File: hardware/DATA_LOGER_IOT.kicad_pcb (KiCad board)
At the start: 2 copper layers, 50 x 50 mm, 9 parts

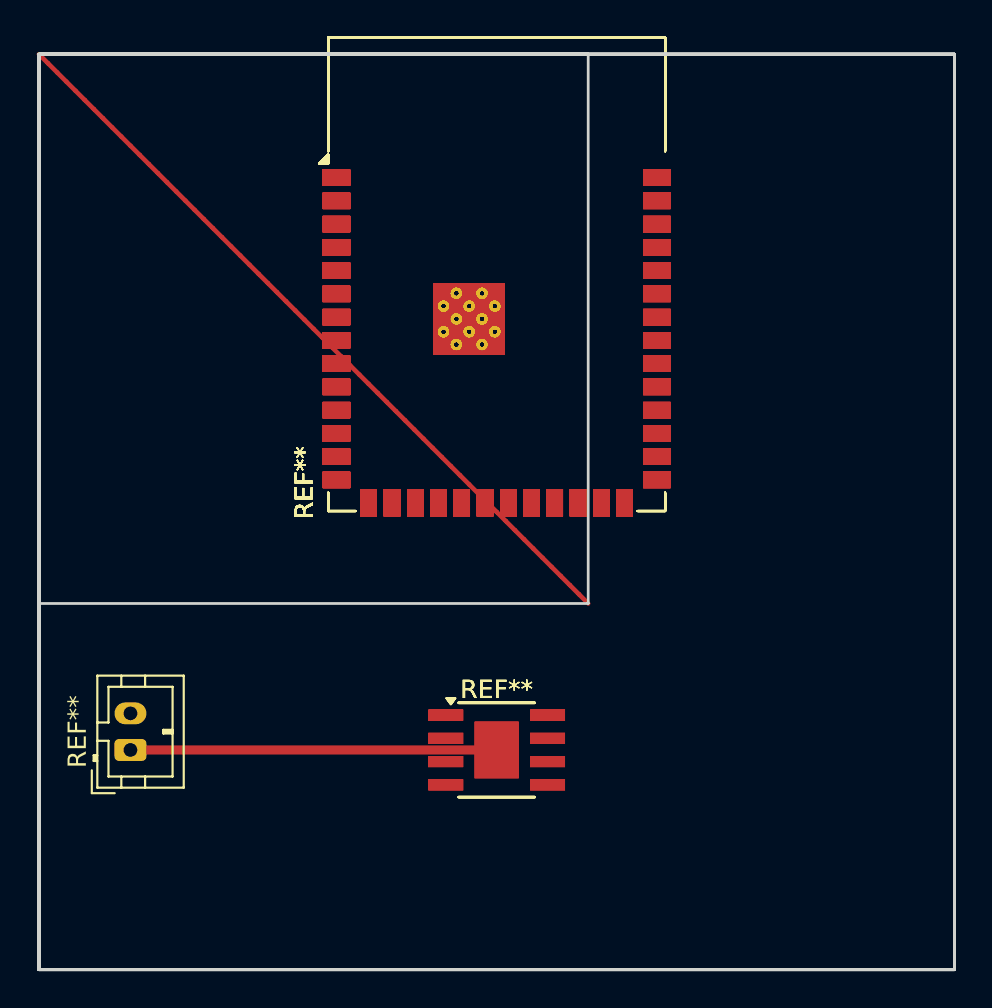
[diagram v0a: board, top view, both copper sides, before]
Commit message: WIP: guardar cambios antes de pull
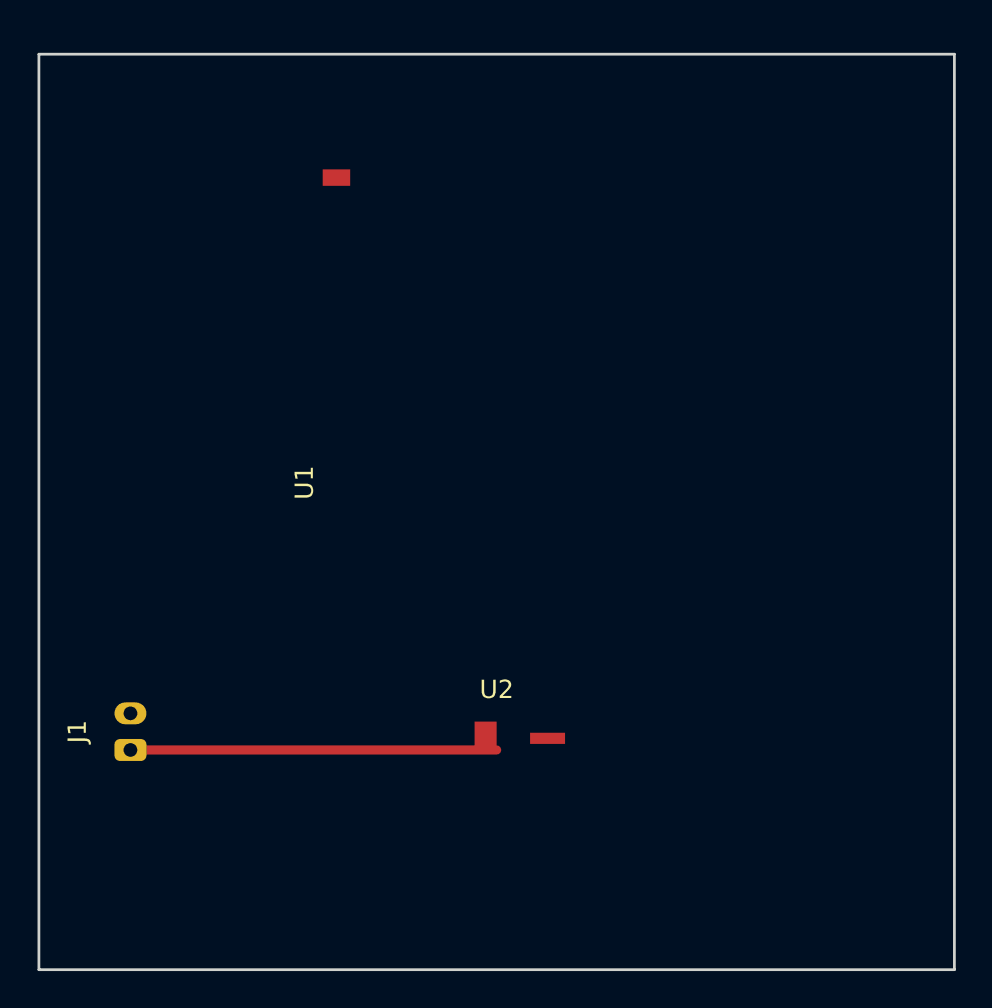
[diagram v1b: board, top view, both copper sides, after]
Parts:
- removed REF** (x5): ESP32-S3-WROOM-1, ESP32-S3-WROOM-1
- removed REF**: TI_SO-PowerPAD-8, TI_SO-PowerPAD-8
- J1: renamed from REF**; value JST_PH_B2B-PH-K_1x02_P2.00mm_Vertical -> (none)
- U1: renamed from REF**; value ESP32-S3-WROOM-1 -> ESP32-S3
- U2: renamed from REF**; value TI_SO-PowerPAD-8 -> (none)
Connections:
- J1 pad 1: (no net) -> +12V
- J1 pad 2: (no net) -> GND
- U2 pad 7: (no net) -> +12V
- U2 pad 9: (no net) -> GND
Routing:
- net (no net): track 42.4 -> 0.00 mm
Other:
- outline, holes or cut-outs redrawn
- net class Power removed
